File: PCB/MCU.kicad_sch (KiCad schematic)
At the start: 27 parts, among them J1 SWD, SW65 Settings, SW66 Reset, U2 W25Q128JVS, U3 RP2040, Y1 12MHz

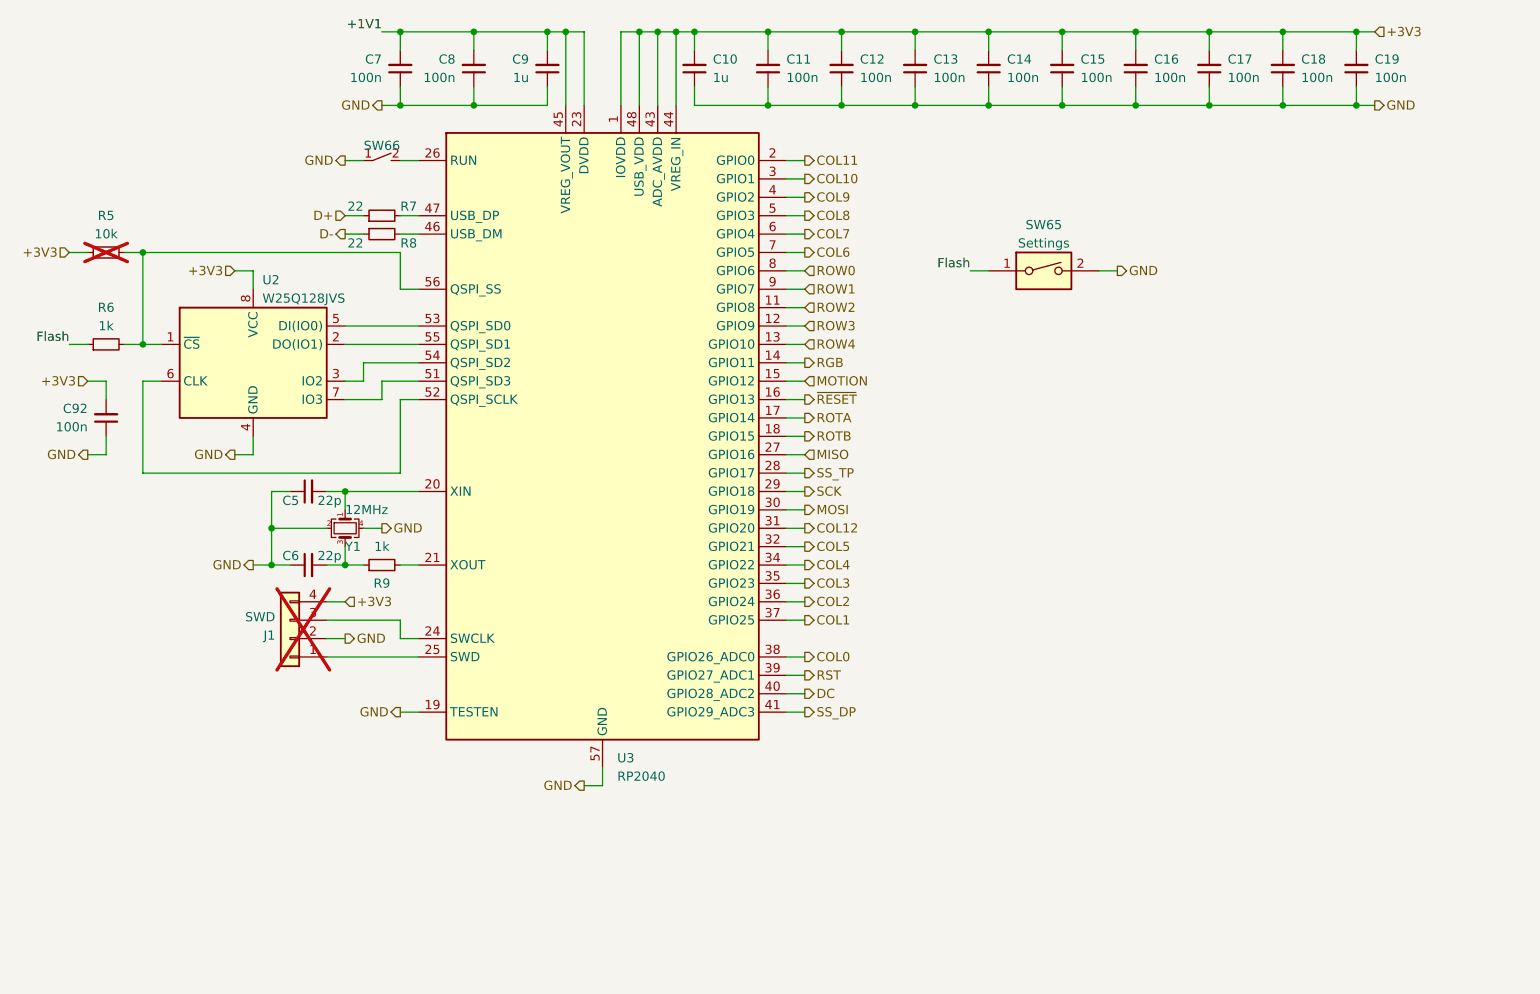
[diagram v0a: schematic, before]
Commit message: Massive mistake corrections and clarifications.
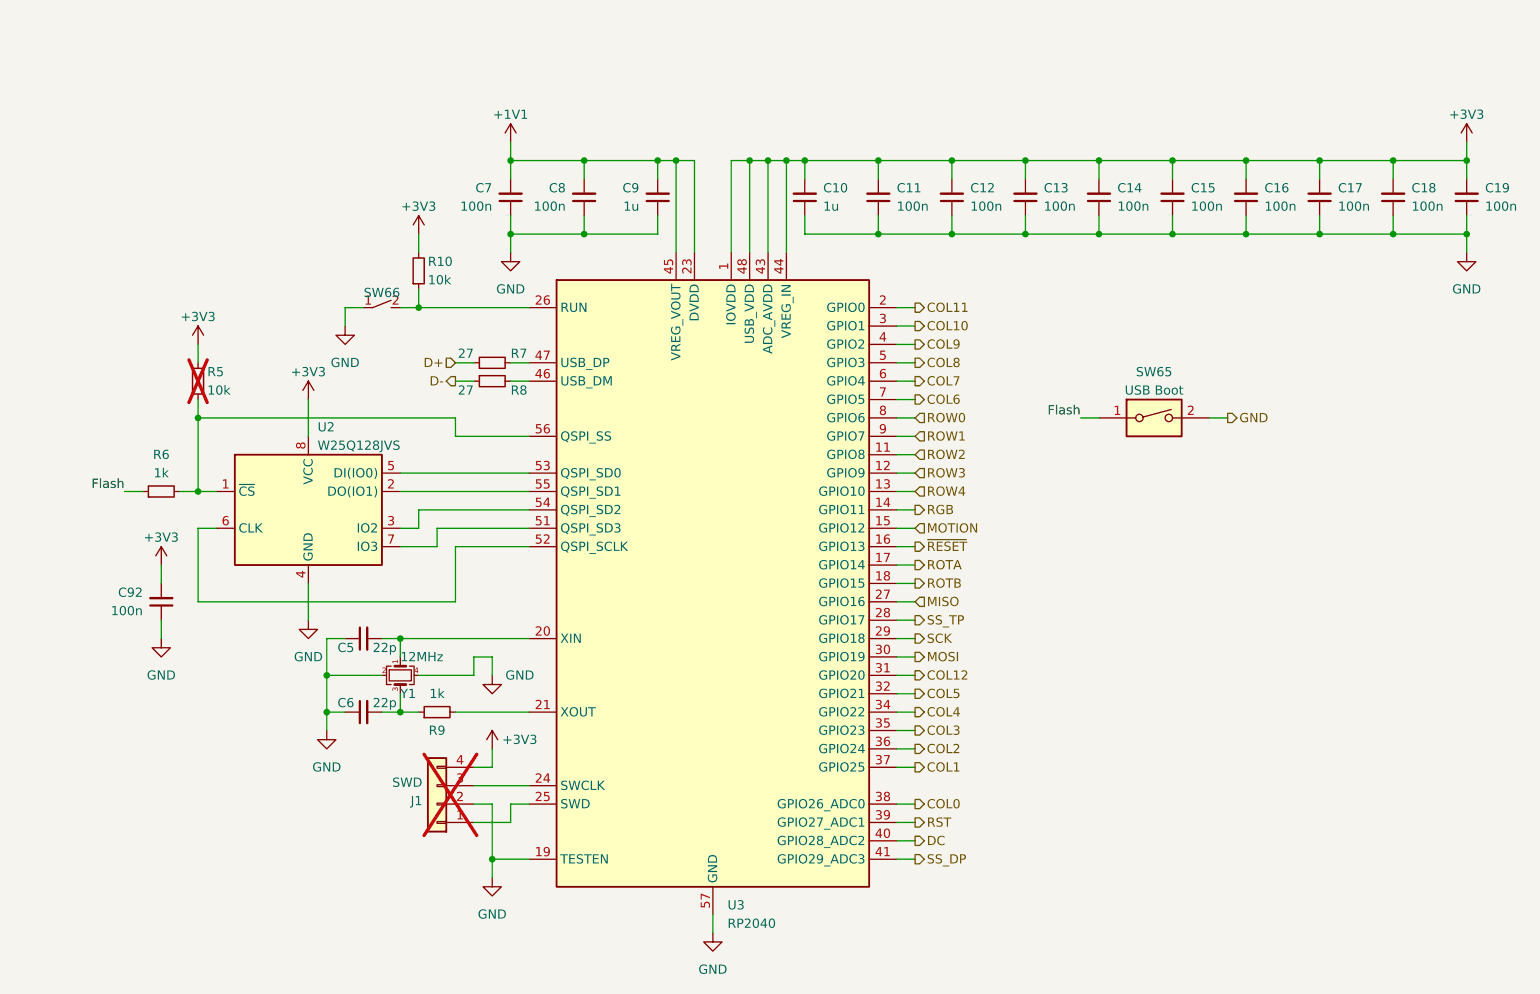
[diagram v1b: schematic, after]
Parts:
- added R10: 10k, Resistor_SMD:R_0402_1005Metric, symbol Device:R_Small
- R7, R8: value 22 -> 27; LCSC part number C25092 -> C25100
- SW65: value Settings -> USB Boot
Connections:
- net +3V3: now also R10.2
- net at SW66.2 (B), U3.26 (RUN): now also R10.1
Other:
- moved on the sheet: C10, C11, C12, C13, C14, C15, C16, C17, C18, C19, C5, C6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
